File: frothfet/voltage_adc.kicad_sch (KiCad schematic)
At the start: 4 parts, among them U23 ADS1015IDGS

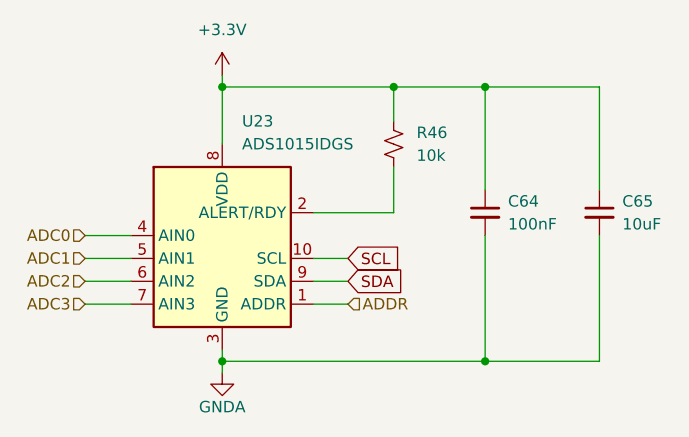
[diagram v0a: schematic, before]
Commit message: prep for new HierarchialPCB test
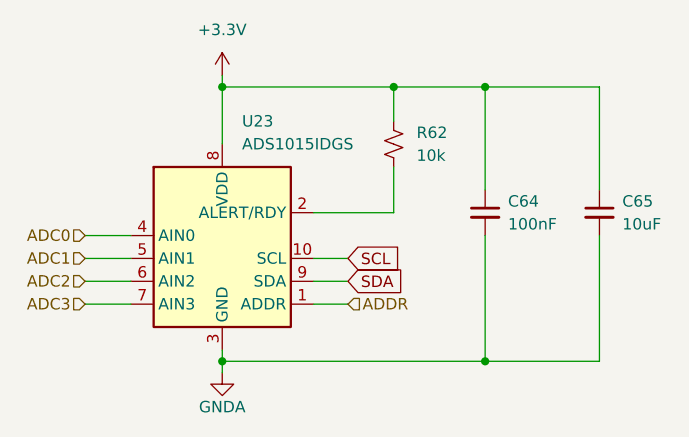
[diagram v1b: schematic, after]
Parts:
- renumbered R46 to R62
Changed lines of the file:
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@@
 		(dnp no)
 		(fields_autoplaced yes)
-		(property "Reference" "R46"
+		(property "Reference" "R62"
 			(at 160.02 82.55 0)
 			(effects
@@
 			(project "8ch-mosfet"
 				(path "/c83c6236-96e9-46ad-9d7a-9e2efa4a7966/a6260305-24e3-4714-b441-a7a157c17bd9"
-					(reference "R46")
+					(reference "R62")
 					(unit 1)
 				)
 				(path "/c83c6236-96e9-46ad-9d7a-9e2efa4a7966/bb9dea8b-8412-49bc-950d-dce57727bcd2"
-					(reference "R45")
+					(reference "R61")
 					(unit 1)
 				)
@@
 		(on_board yes)
 		(dnp no)
-		(property "Reference" "#PWR072"
+		(property "Reference" "#PWR080"
 			(at 138.43 115.57 0)
 			(effects
@@
 			(project "8ch-mosfet"
 				(path "/c83c6236-96e9-46ad-9d7a-9e2efa4a7966/a6260305-24e3-4714-b441-a7a157c17bd9"
-					(reference "#PWR072")
+					(reference "#PWR080")
 					(unit 1)
 				)
 				(path "/c83c6236-96e9-46ad-9d7a-9e2efa4a7966/bb9dea8b-8412-49bc-950d-dce57727bcd2"
-					(reference "#PWR070")
+					(reference "#PWR078")
 					(unit 1)
 				)
@@
 		(dnp no)
 		(fields_autoplaced yes)
-		(property "Reference" "#PWR071"
+		(property "Reference" "#PWR079"
 			(at 138.43 80.01 0)
 			(effects
@@
 			(project "8ch-mosfet"
 				(path "/c83c6236-96e9-46ad-9d7a-9e2efa4a7966/a6260305-24e3-4714-b441-a7a157c17bd9"
-					(reference "#PWR071")
+					(reference "#PWR079")
 					(unit 1)
 				)
 				(path "/c83c6236-96e9-46ad-9d7a-9e2efa4a7966/bb9dea8b-8412-49bc-950d-dce57727bcd2"
-					(reference "#PWR069")
-					(unit 1)
-				)
+					(reference "#PWR077")
+					(unit 1)
+				)
